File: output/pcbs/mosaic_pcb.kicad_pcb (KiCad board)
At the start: 2 copper layers, 100 x 95 mm, 20 parts

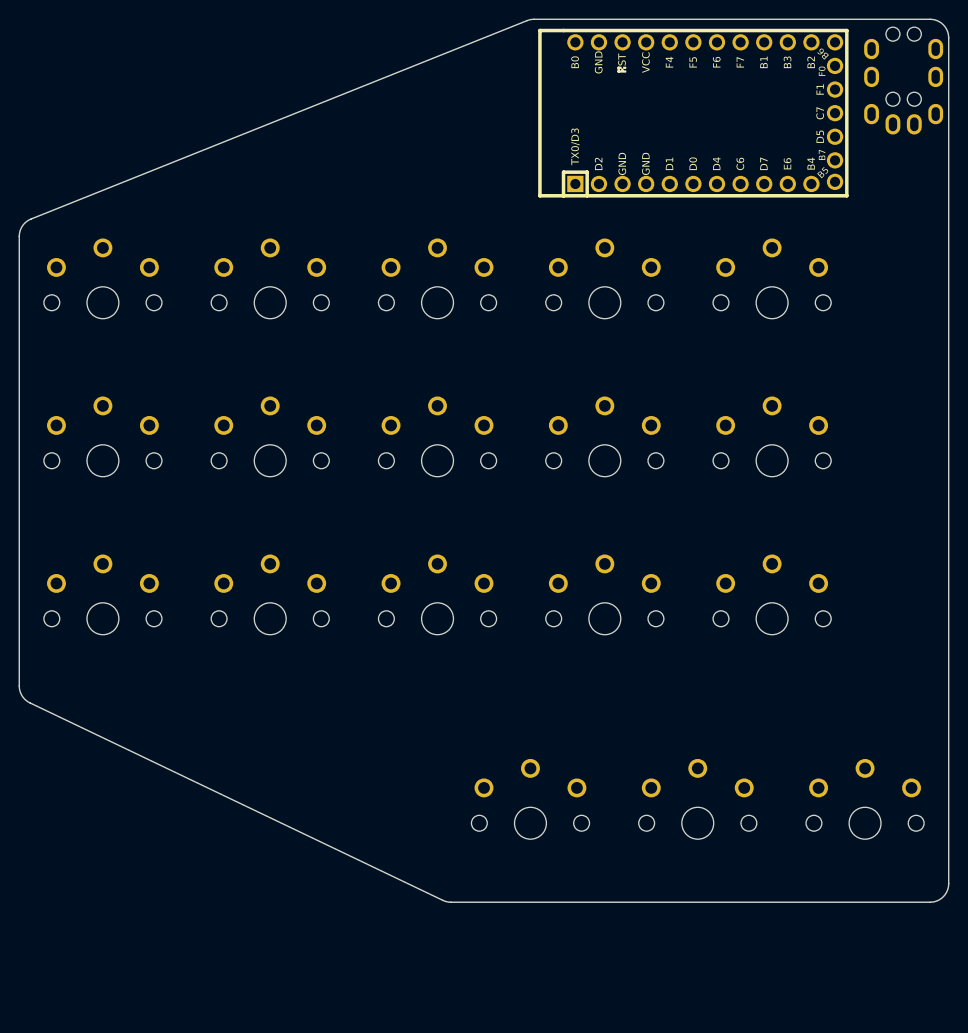
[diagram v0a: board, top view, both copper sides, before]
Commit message: mosaic v0.0.1 (#1)
* rp2040 zero,diodeless, hotswap
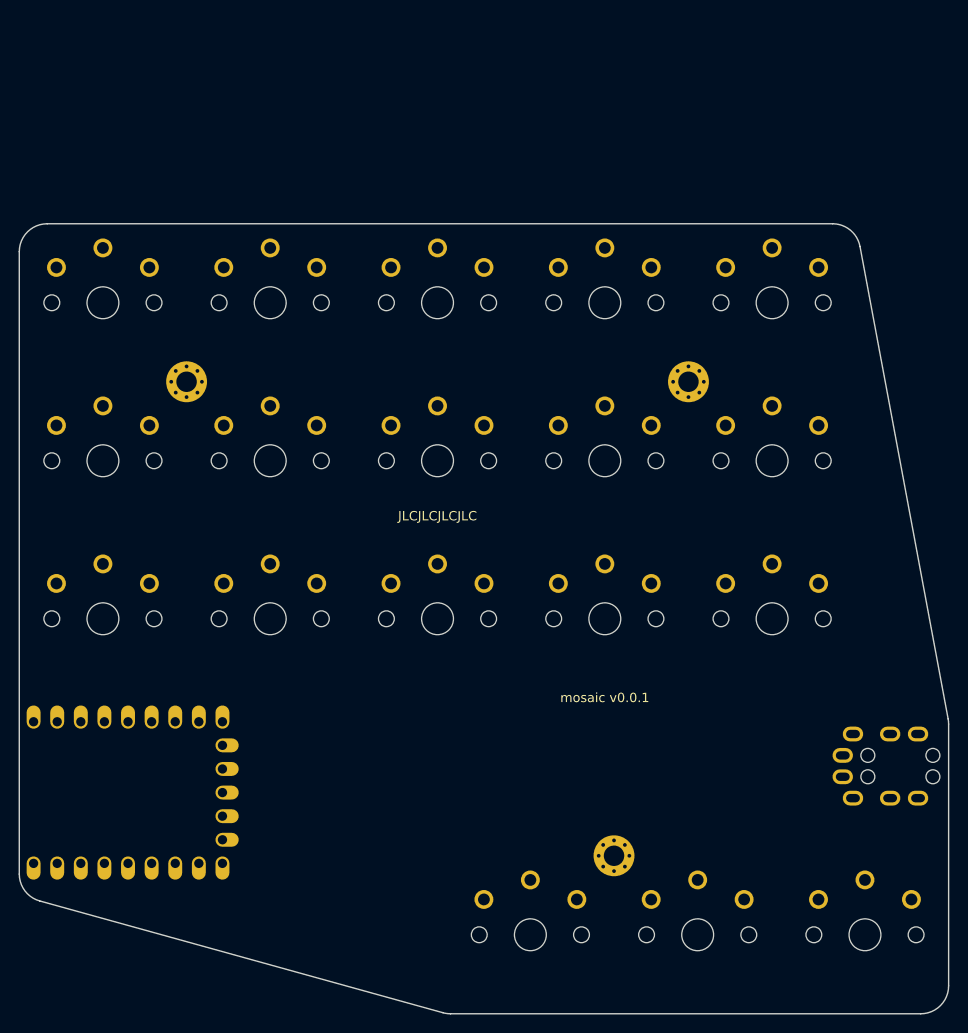
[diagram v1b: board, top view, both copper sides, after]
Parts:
- removed the ? at (208.8, 81.6)
- added ?: , rp2040_zero_tht_pads, F.Cu at (146.7, 154.7)
- added _2: , MountingHole_2.2mm_M2_Pad_Via, F.Cu at (153.0, 110.5)
- added _3: , MountingHole_2.2mm_M2_Pad_Via, F.Cu at (199.0, 161.5)
- added _4: , MountingHole_2.2mm_M2_Pad_Via, F.Cu at (207.0, 110.5)
- moved TRRS1 81.6 mm to (234.9, 153.0), turned to 270 degrees
- moved S16 12.0 mm to (190.0, 170.0)
- moved S17 12.0 mm to (208.0, 170.0)
- moved S18 12.0 mm to (226.0, 170.0)
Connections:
- TRRS1 pad 1: GND -> 3V3
- TRRS1 pad 2: VCC -> GND
- TRRS1 pad 3: D3 -> GP9
- TRRS1 pad 4: D2 -> GP8
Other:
- board size 100 x 95 mm -> 100 x 85 mm
- board text added: "JLCJLCJLCJLC"
- board text added: "mosaic v0.0.1"
